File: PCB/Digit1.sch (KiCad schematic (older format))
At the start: 1 part

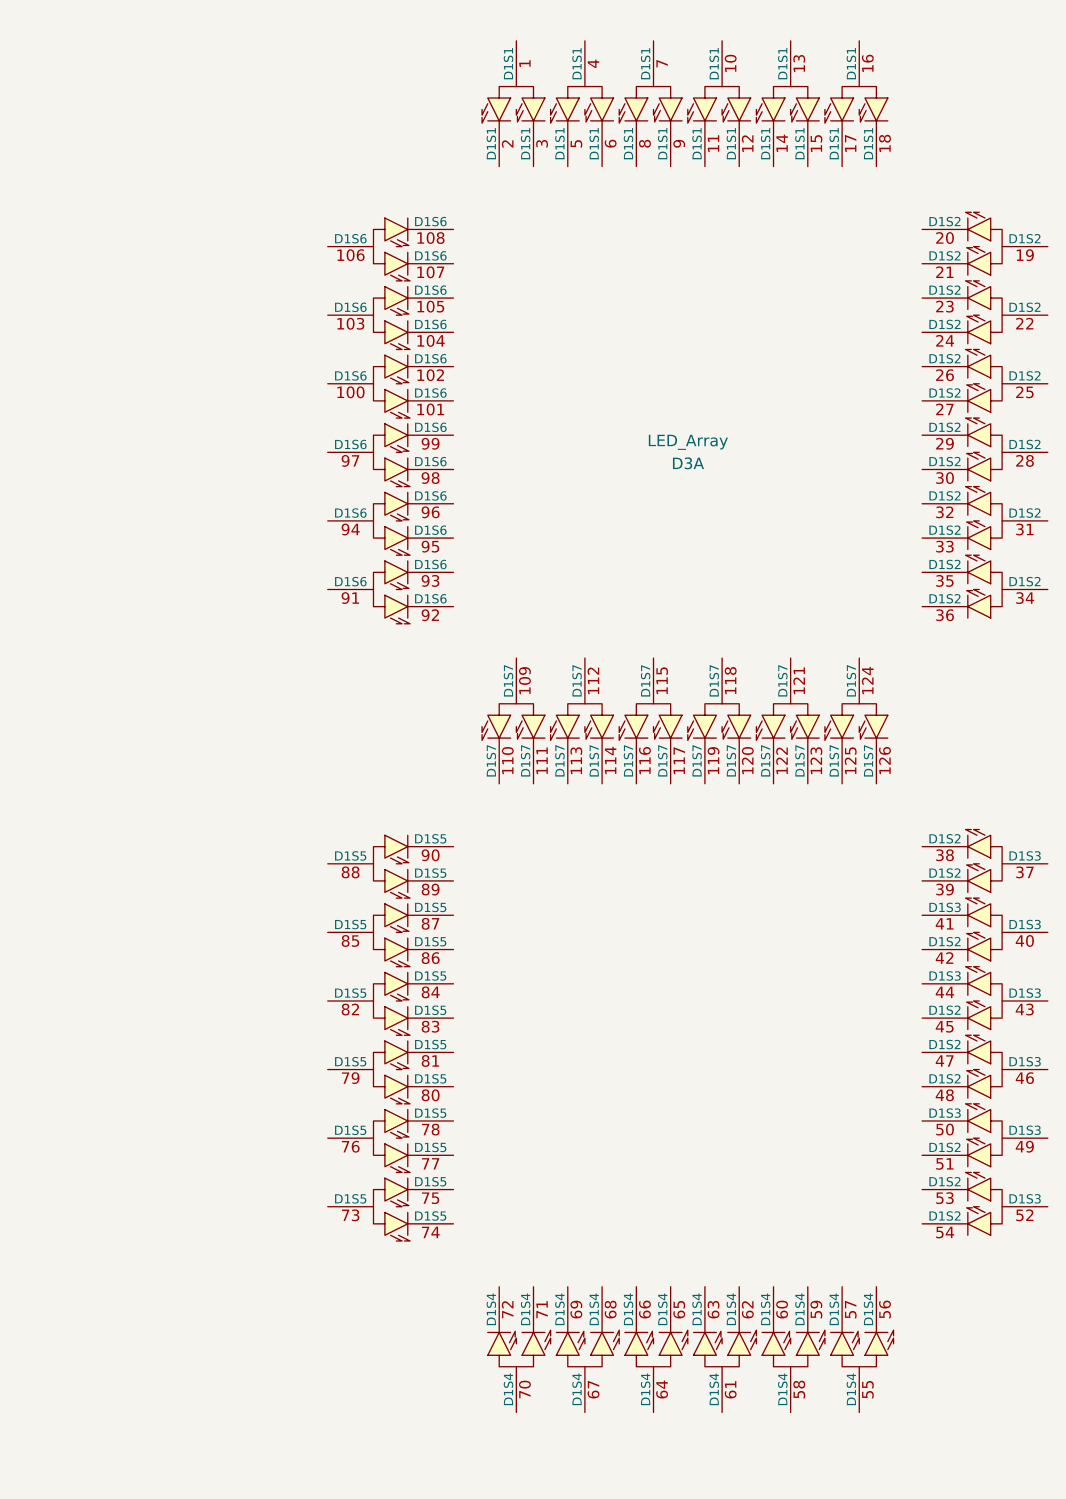
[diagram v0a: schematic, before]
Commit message: Worked on PCB.
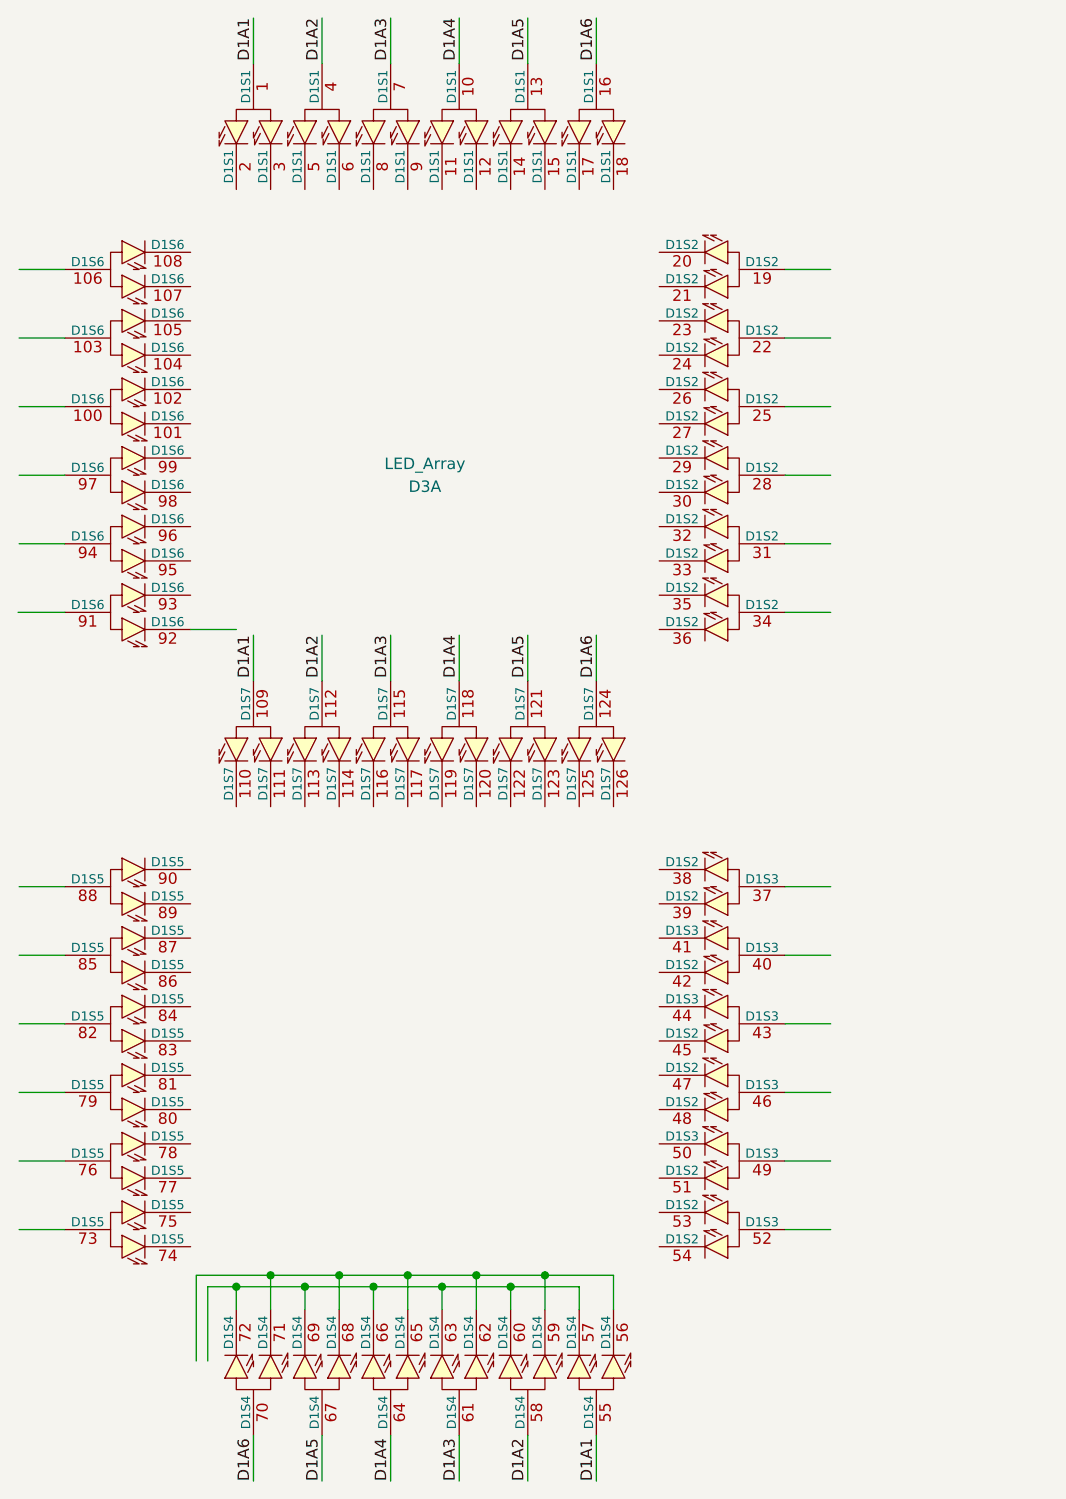
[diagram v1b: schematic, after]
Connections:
- net labels added: D1A1, D1A2, D1A3, D1A4, D1A5, D1A6
- wire segments 0 -> 59
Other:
- moved on the sheet: D3A
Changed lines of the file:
@@
 Comment4 ""
 $EndDescr
+Text Label 3000 950  3    50   ~ 0
+D1A1
+Text Label 3300 950  3    50   ~ 0
+D1A2
+Text Label 3600 950  3    50   ~ 0
+D1A3
+Text Label 3900 950  3    50   ~ 0
+D1A4
+Text Label 4200 950  3    50   ~ 0
+D1A5
+Text Label 4500 950  3    50   ~ 0
+D1A6
+Text Label 3000 3650 3    50   ~ 0
+D1A1
+Text Label 3300 3650 3    50   ~ 0
+D1A2
+Text Label 3600 3650 3    50   ~ 0
+D1A3
+Text Label 3900 3650 3    50   ~ 0
+D1A4
+Text Label 4200 3650 3    50   ~ 0
+D1A5
+Text Label 4500 3650 3    50   ~ 0
+D1A6
+Text Label 4500 7350 1    50   ~ 0
+D1A1
+Text Label 4200 7350 1    50   ~ 0
+D1A2
+Text Label 3900 7350 1    50   ~ 0
+D1A3
+Text Label 3600 7350 1    50   ~ 0
+D1A4
+Text Label 3300 7350 1    50   ~ 0
+D1A5
+Text Label 3000 7350 1    50   ~ 0
+D1A6
 $Comp
 L LED_Array D3
 U 1 1 54BC75FA
-P 4900 4050
-F 0 "D3" H 4900 5200 50  0000 C CNN
-F 1 "LED_Array" H 4900 5300 50  0000 C CNN
-F 2 "Custom:LED-ARRAY" H 4900 4975 50  0001 C CNN
-F 3 "" H 4900 4975 50  0000 C CNN
-	1    4900 4050
+P 3750 4150
+F 0 "D3" H 3750 5300 50  0000 C CNN
+F 1 "LED_Array" H 3750 5400 50  0000 C CNN
+F 2 "Custom:LED-ARRAY" H 3750 5075 50  0001 C CNN
+F 3 "" H 3750 5075 50  0000 C CNN
+	1    3750 4150
 	1    0    0    -1
 $EndComp
+Wire Wire Line
+	3000 1150 3000 950
+Wire Wire Line
+	3300 1150 3300 950
+Wire Wire Line
+	3600 1150 3600 950
+Wire Wire Line
+	3900 1150 3900 950
+Wire Wire Line
+	4200 1150 4200 950
+Wire Wire Line
+	4500 1150 4500 950
+Wire Wire Line
+	5325 2350 5525 2350
+Wire Wire Line
+	5325 2050 5525 2050
+Wire Wire Line
+	5325 2650 5525 2650
+Wire Wire Line
+	5325 2950 5525 2950
+Wire Wire Line
+	5325 3250 5525 3250
+Wire Wire Line
+	5325 3550 5525 3550
+Wire Wire Line
+	5325 4750 5525 4750
+Wire Wire Line
+	5325 5050 5525 5050
+Wire Wire Line
+	5325 5350 5525 5350
+Wire Wire Line
+	5325 5650 5525 5650
+Wire Wire Line
+	5325 5950 5525 5950
+Wire Wire Line
+	5325 6250 5525 6250
+Wire Wire Line
+	4500 7150 4500 7350
+Wire Wire Line
+	4200 7150 4200 7350
+Wire Wire Line
+	3900 7150 3900 7350
+Wire Wire Line
+	3600 7150 3600 7350
+Wire Wire Line
+	3300 7150 3300 7350
+Wire Wire Line
+	3000 7150 3000 7350
+Wire Wire Line
+	2175 6250 1975 6250
+Wire Wire Line
+	2175 5950 1975 5950
+Wire Wire Line
+	2175 5650 1975 5650
+Wire Wire Line
+	2175 5350 1975 5350
+Wire Wire Line
+	2175 5050 1975 5050
+Wire Wire Line
+	2175 4750 1975 4750
+Wire Wire Line
+	2175 3550 1970 3550
+Wire Wire Line
+	2175 3250 1975 3250
+Wire Wire Line
+	2175 2950 1975 2950
+Wire Wire Line
+	2175 2650 1975 2650
+Wire Wire Line
+	2175 2350 1975 2350
+Wire Wire Line
+	2175 2050 1975 2050
+Wire Wire Line
+	3000 3850 3000 3650
+Wire Wire Line
+	3300 3850 3300 3650
+Wire Wire Line
+	3600 3850 3600 3650
+Wire Wire Line
+	3900 3850 3900 3650
+Wire Wire Line
+	4200 3850 4200 3650
+Wire Wire Line
+	4500 3850 4500 3650
+Wire Wire Line
+	2725 3625 2925 3625
+Wire Wire Line
+	4425 6500 4425 6600
+Wire Wire Line
+	2800 6500 4425 6500
+Wire Wire Line
+	2800 6500 2800 6825
+Wire Wire Line
+	4125 6600 4125 6500
+Connection ~ 4125 6500
+Wire Wire Line
+	3825 6600 3825 6500
+Connection ~ 3825 6500
+Wire Wire Line
+	3525 6600 3525 6500
+Connection ~ 3525 6500
+Wire Wire Line
+	3225 6600 3225 6500
+Connection ~ 3225 6500
+Wire Wire Line
+	2925 6600 2925 6500
+Connection ~ 2925 6500
+Wire Wire Line
+	4575 6600 4575 6450
+Wire Wire Line
+	4575 6450 2750 6450
+Wire Wire Line
+	2750 6450 2750 6825
+Wire Wire Line
+	4275 6600 4275 6450
+Connection ~ 4275 6450
+Wire Wire Line
+	3975 6600 3975 6450
+Connection ~ 3975 6450
+Wire Wire Line
+	3675 6600 3675 6450
+Connection ~ 3675 6450
+Wire Wire Line
+	3375 6600 3375 6450
+Connection ~ 3375 6450
+Wire Wire Line
+	3075 6600 3075 6450
+Connection ~ 3075 6450
 $EndSCHEMATC
